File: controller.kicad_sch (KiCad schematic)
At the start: 34 parts, among them J1 Conn_ST_STDC14, J2 USB_C_Receptacle_USB2.0_14P, SW1 SW_Push, SW2 SW_Push, SW3 SW_Push, SW4 SW_Push, SW5 SW_Push, SW6 SW_Push, U1 STM32L476RGTx, U2 BD33FC0FP, U3 NUP2202

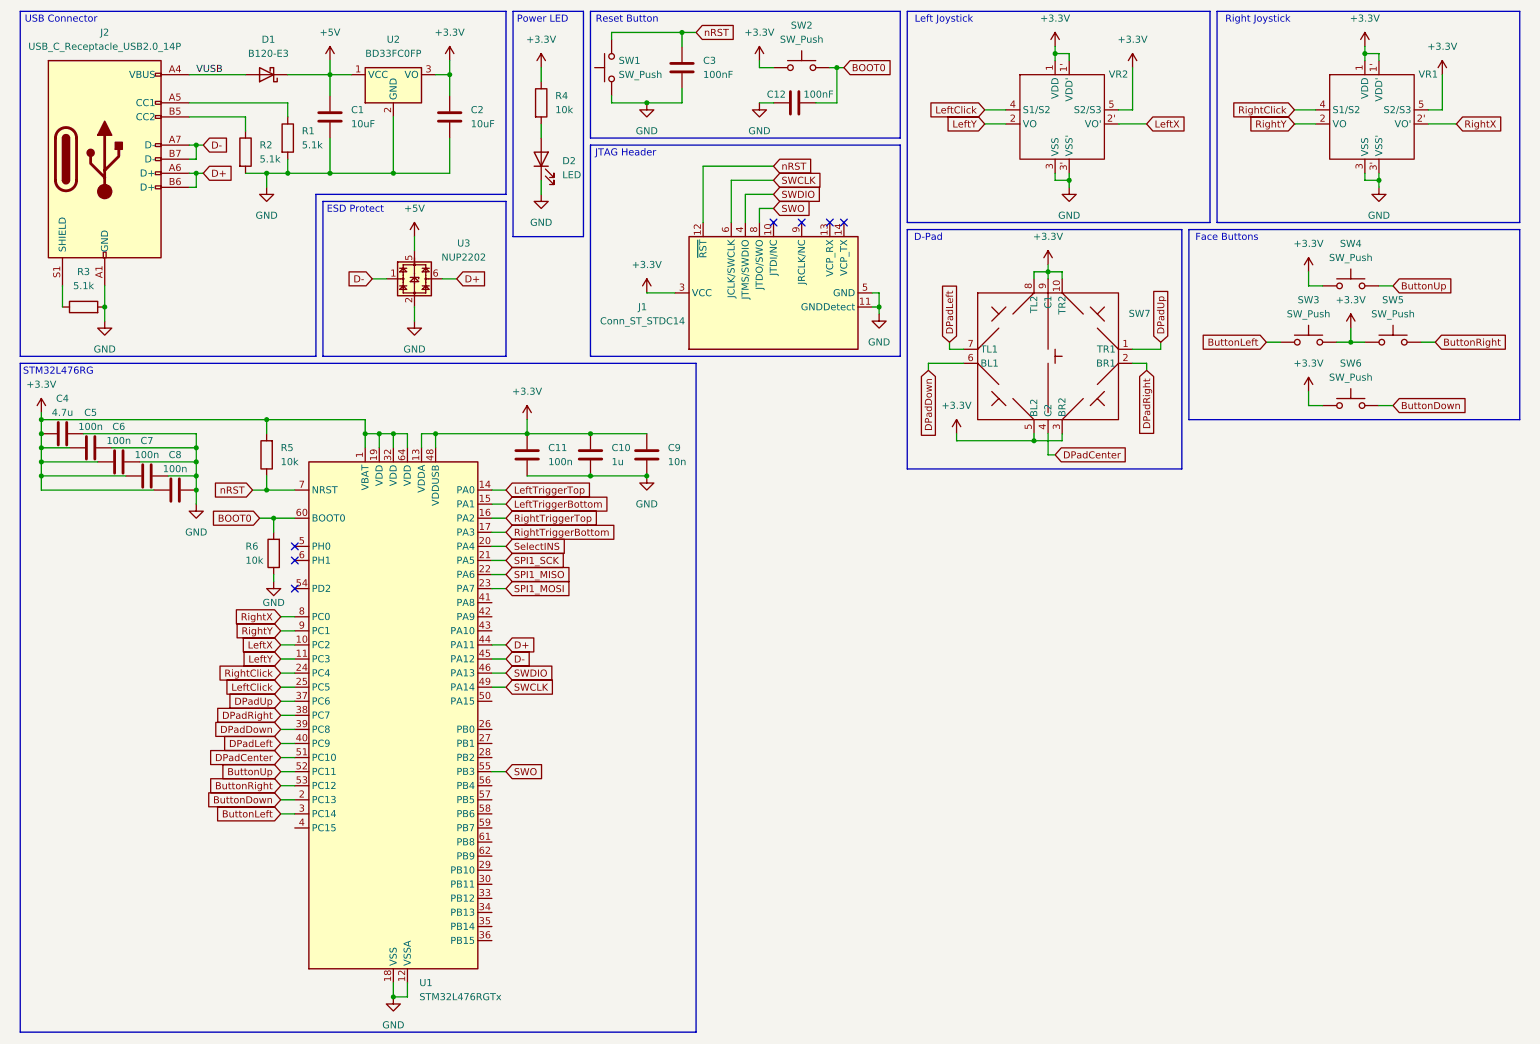
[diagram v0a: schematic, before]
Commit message: finish routing, more or less
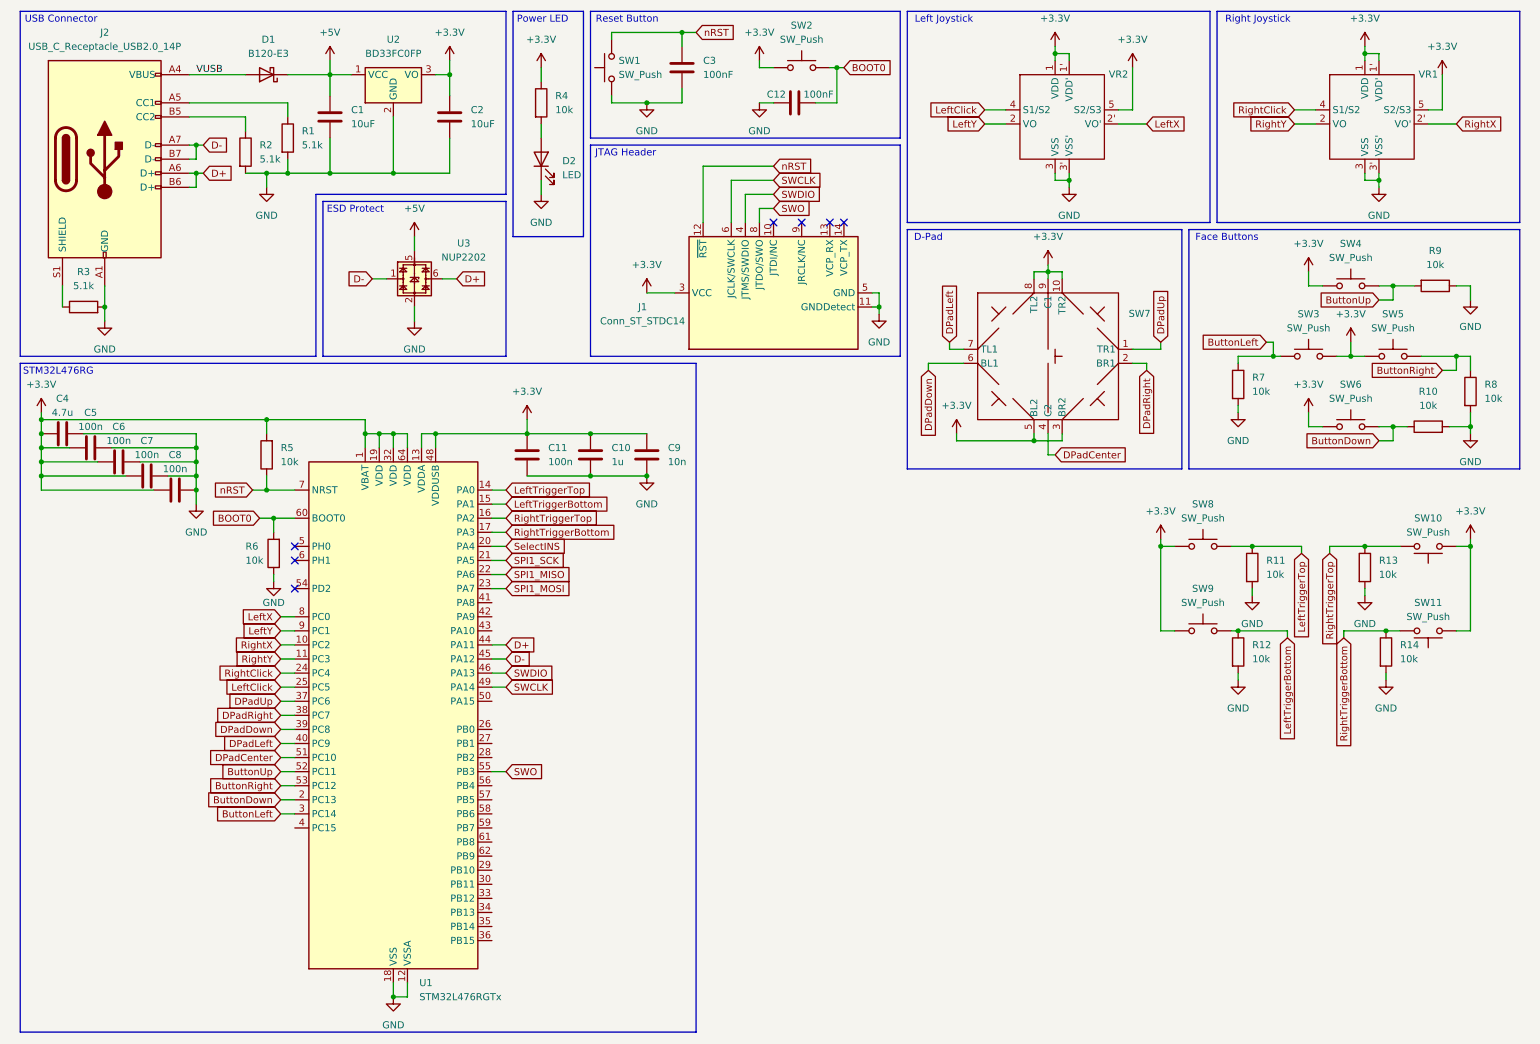
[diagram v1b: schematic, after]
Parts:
- added R10, R11, R12, R13, R14, R7, R8, R9: 10k, Resistor_SMD:R_0201_0603Metric, symbol Device:R
- added SW10, SW11, SW8, SW9: SW_Push, Button_Switch_SMD:SW_Push_1P1T-MP_NO_Horizontal_Alps_SKRTLAE010, symbol Switch:SW_Push
- SW3, SW4, SW5, SW6: footprint (none) -> Button_Switch_SMD:SW_Push_1P1T_NO_CK_PTS125Sx43SMTR
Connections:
- net +3.3V: now also SW10.1, SW11.1, SW8.1, SW9.1
- net ButtonDown: now also R10.1
- net ButtonLeft: now also R7.1
- net ButtonRight: now also R8.1
- net ButtonUp: now also R9.2
- net GND: now also R10.2, R11.2, R12.2, R13.2, R14.2, R7.2, R8.2, R9.1
- net LeftTriggerBottom: now also R12.1, SW9.2
- net LeftTriggerTop: now also R11.1, SW8.2
- net LeftX: now also U1.8 (PC0); no longer U1.10 (PC2)
- net LeftY: now also U1.9 (PC1); no longer U1.11 (PC3)
- net RightTriggerBottom: now also R14.1, SW11.2
- net RightTriggerTop: now also R13.1, SW10.2
- net RightX: now also U1.10 (PC2); no longer U1.8 (PC0)
- net RightY: now also U1.11 (PC3); no longer U1.9 (PC1)
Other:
- moved on the sheet: SW3, SW5, SW6
